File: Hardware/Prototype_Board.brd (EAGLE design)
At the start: 117.8 x 92.7 mm, 11 parts

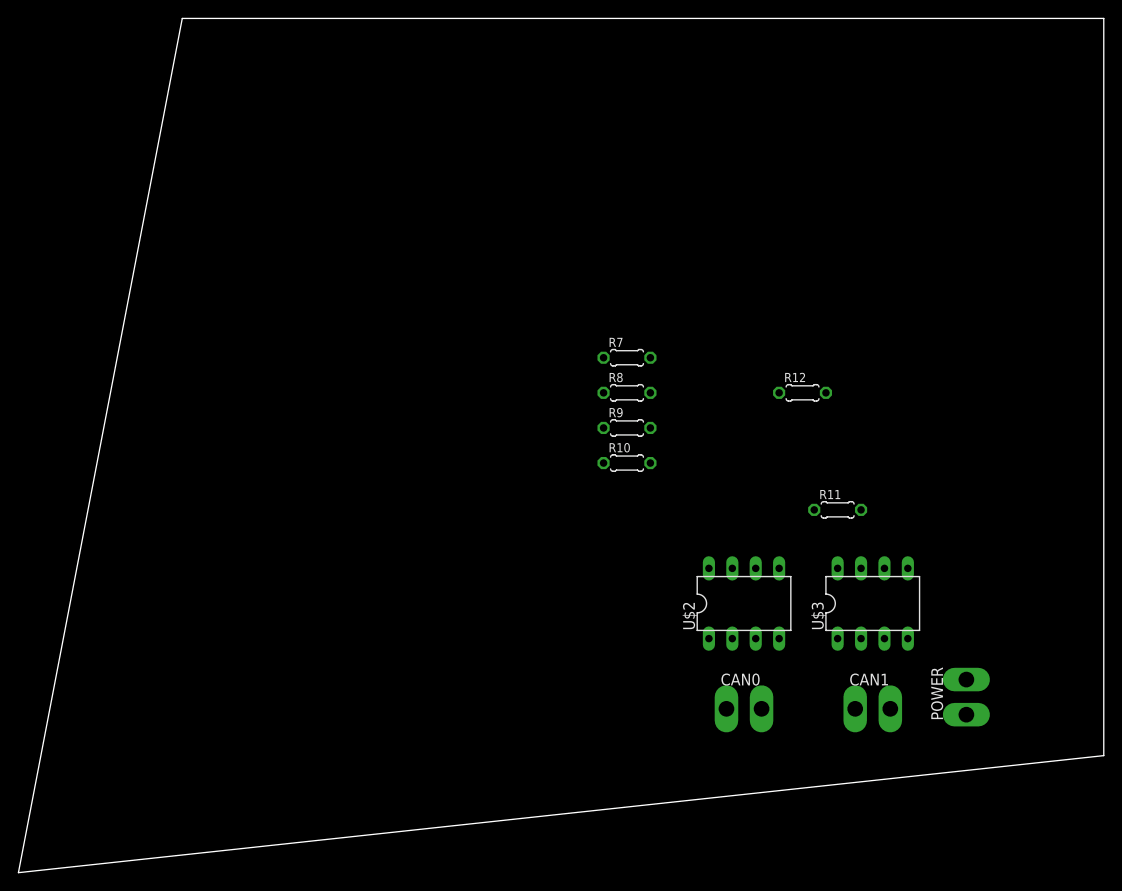
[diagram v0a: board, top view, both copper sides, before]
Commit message: Prototype Board & Schematic
This is the updated board and schematic for the prototype
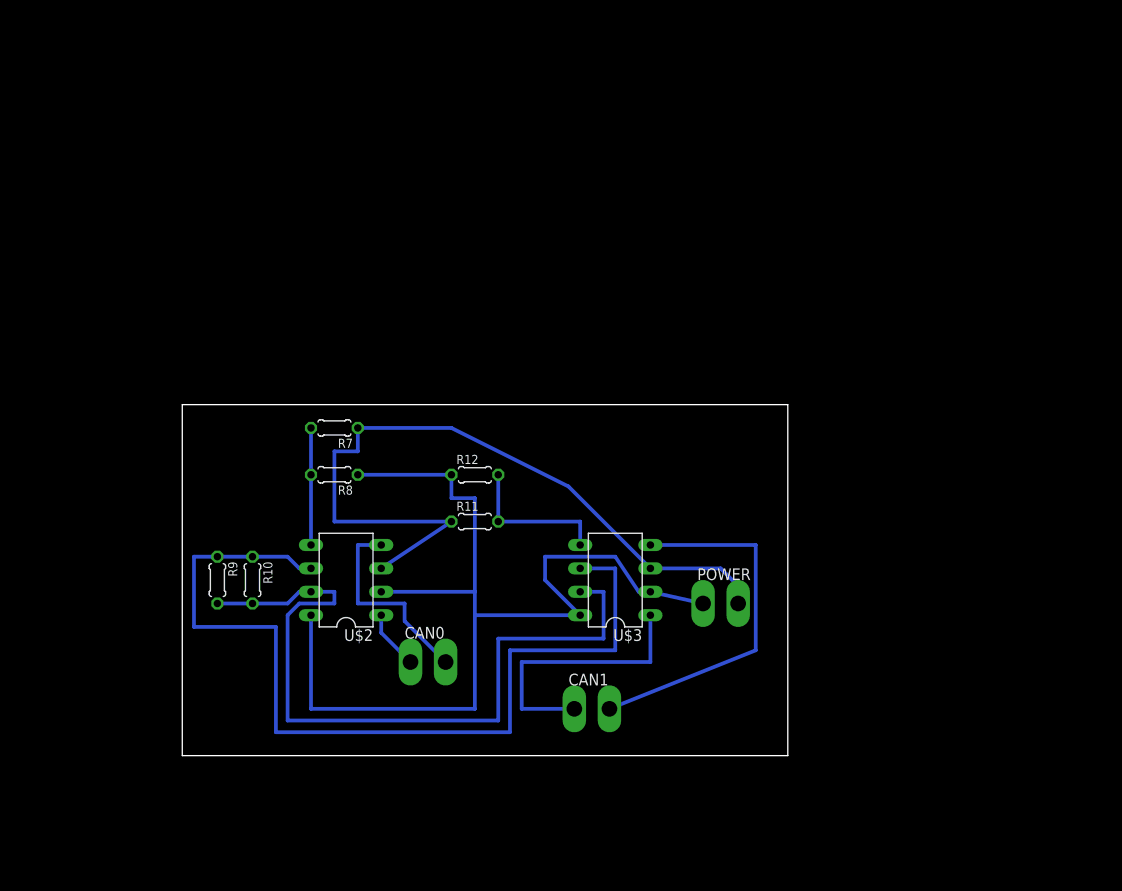
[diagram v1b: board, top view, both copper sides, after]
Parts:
- moved R9 47.4 mm to (3.81, 19.1), turned to 270 degrees
- moved U$2 43.3 mm to (17.8, 19.1), turned to 90 degrees
- moved R10 42.6 mm to (7.62, 19.1), turned to 270 degrees
- moved R11 39.4 mm to (31.8, 25.4)
- moved R12 36.7 mm to (31.8, 30.5)
- moved CAN0 34.7 mm to (26.7, 10.2)
- moved R8 33.0 mm to (16.5, 30.5), turned to 180 degrees
- moved R7 32.7 mm to (16.5, 35.6), turned to 180 degrees
- moved CAN1 30.5 mm to (44.5, 5.08)
- moved POWER 28.5 mm to (58.4, 16.5), turned to 0 degrees
- moved U$3 28.1 mm to (47.0, 19.1), turned to 90 degrees
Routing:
- net GND: track 0.00 -> 114.9 mm
- net N$8: track 0.00 -> 99.6 mm
- net VCC: track 0.00 -> 83.7 mm
- net N$4: track 0.00 -> 82.3 mm
- net RX2: track 0.01 -> 40.0 mm
- net TX2: track 0.00 -> 29.8 mm
- net RX1: track 0.00 -> 22.2 mm
- net N$7: track 0.00 -> 16.5 mm
- net N$3: track 0.00 -> 12.7 mm
- net TX1: track 0.00 -> 6.40 mm
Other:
- board size 117.8 x 92.7 mm -> 65.7 x 38.1 mm
